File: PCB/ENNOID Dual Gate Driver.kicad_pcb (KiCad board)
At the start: 2 copper layers, 60 x 98 mm, 137 parts, among them J1 Conn_02x08_Odd_Even, J2 Current, J3 TEMP, J4 PHASE, J5 Collector, J6 Gate_H, J7 G_L, J8 E, Q1 Q_NPN_BCE, Q2 Q_NPN_BCE, Q3 2N7002K-7, Q4 2N7002K-7, Q5 2N7002, Q6 2N7002, Q7 2N7002, Q8 2N7002, U1 MC7805, U2 MGJ2, U3 MGJ2, U4 1ED020I12-F2, U5 IXD-609, U6 1ED020I12-F2, U7 IXD-609, U8 AMC1301, U9 4069

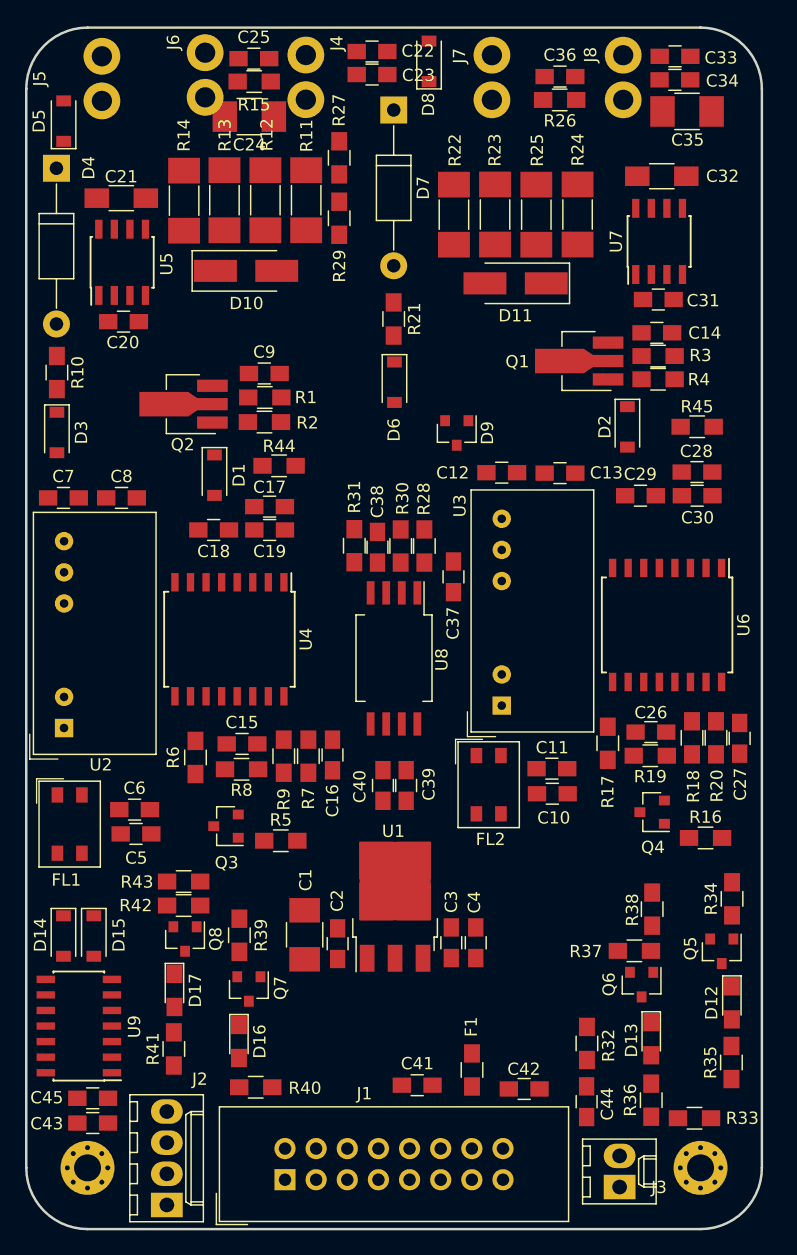
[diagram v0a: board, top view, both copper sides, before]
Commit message: Routing has started
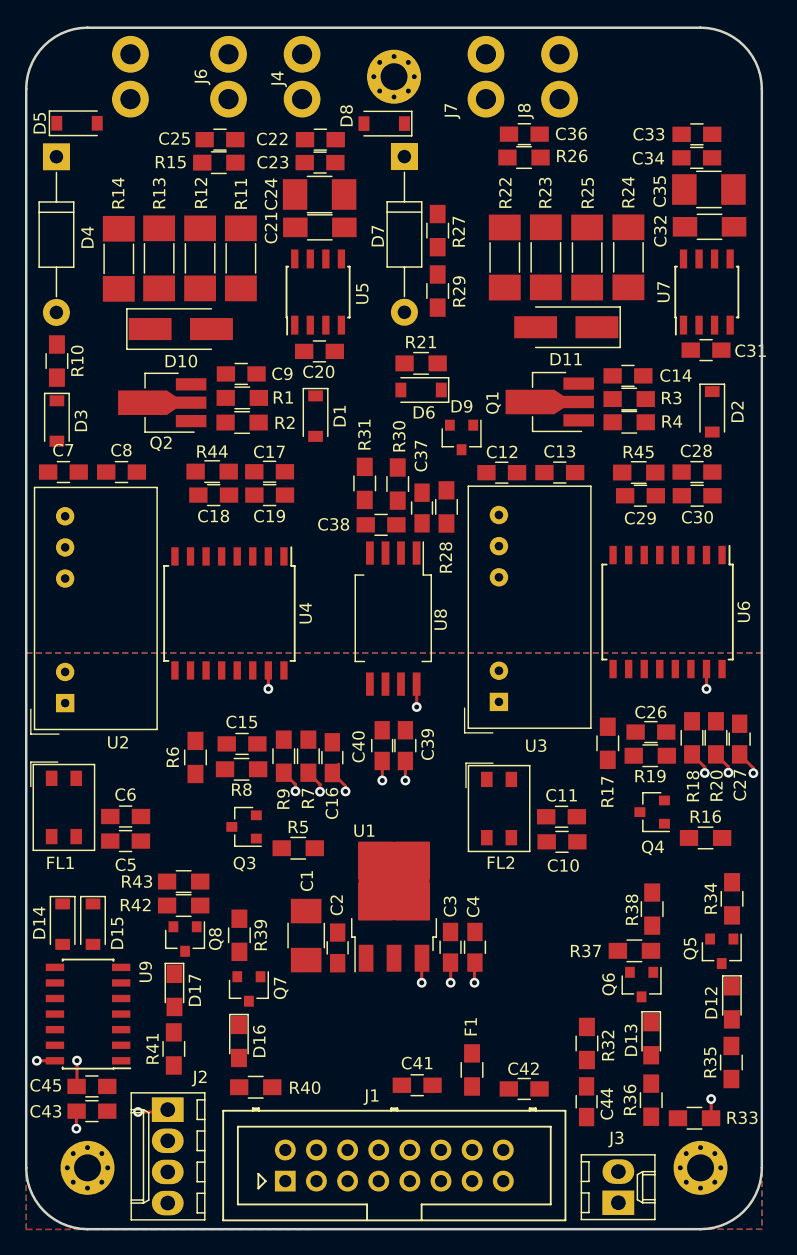
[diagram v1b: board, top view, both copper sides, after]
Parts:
- added REF**: MountingHole_2.2mm_M2_Pad_Via, Mounting_Holes:MountingHole_2.2mm_M2_Pad_Via, F.Cu at (30.0, 4.00)
- J1: footprint Connectors_IDC:IDC-Header_2x08_Pitch2.54mm_Straight -> Connectors_Multicomp:Multicomp_MC9A12-1634_2x08x2.54mm_Straight
- J5: moved to B.Cu
- moved C21 16.4 mm to (23.9, 16.3)
- moved C20 16.2 mm to (23.9, 26.4)
- moved U5 16.2 mm to (23.8, 21.6)
- moved R27 9.99 mm to (33.6, 16.6)
- moved R29 9.99 mm to (33.6, 21.5)
- moved D1 9.55 mm to (23.6, 31.7)
- moved C24 8.56 mm to (23.9, 13.6), turned to 0 degrees
- moved C23 8.34 mm to (24.0, 11.0), turned to 0 degrees
- moved C22 8.34 mm to (24.0, 9.13), turned to 0 degrees
- moved J2 7.77 mm to (11.5, 88.3), turned to 270 degrees
- moved R15 7.22 mm to (15.7, 11.0)
- moved C25 7.16 mm to (15.8, 9.13)
- moved D10 7.13 mm to (12.6, 24.6)
- moved R13 7.13 mm to (10.8, 18.8)
- moved R12 7.13 mm to (14.2, 18.8)
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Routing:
- net +5V: track 0.00 -> 34.9 mm, vias 0 -> 19
- added copper zone on B.Cu, net +5V
- added copper zone on F.Cu, net GND

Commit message: PCB completed with readme update
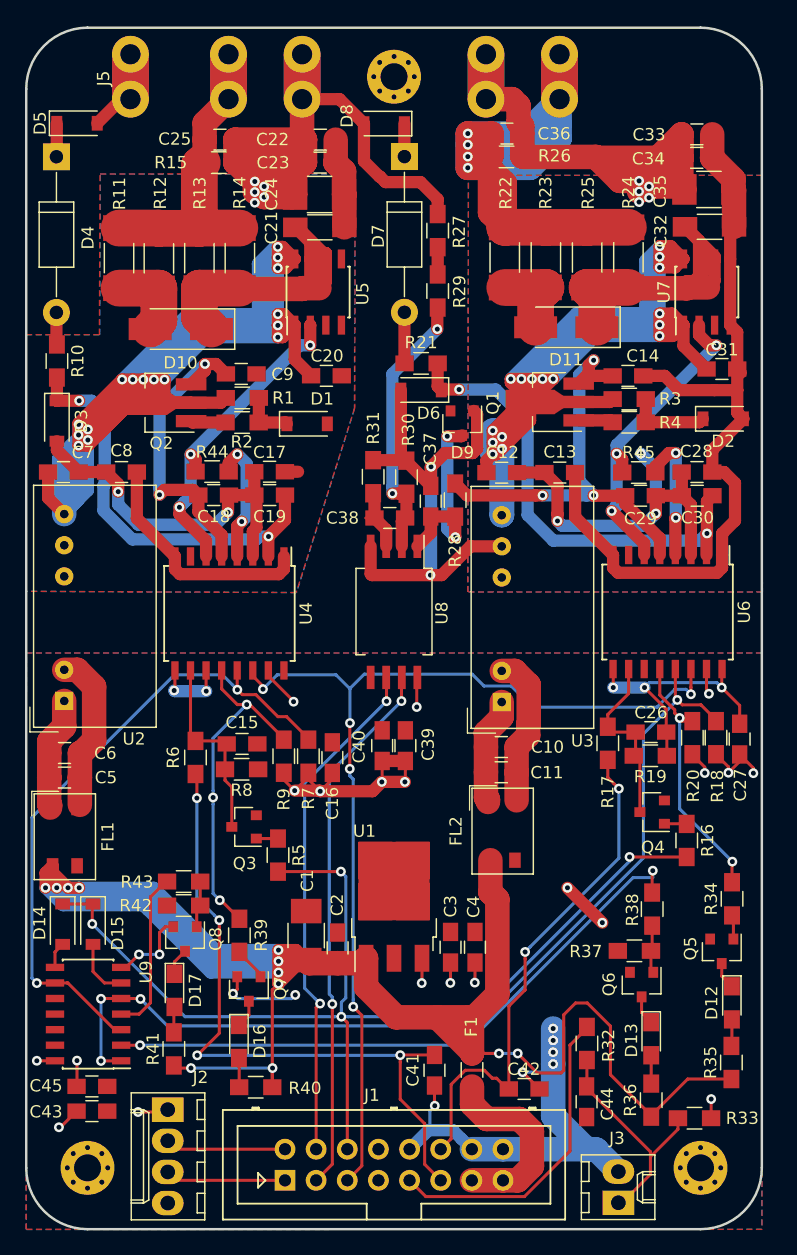
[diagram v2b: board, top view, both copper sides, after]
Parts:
- FL1, FL2: value ACM4520-142-2P-T000 -> ACM4520
- J1: footprint Connectors_Multicomp:Multicomp_MC9A12-1634_2x08x2.54mm_Straight -> ENNOID:Multicomp_MC9A12-1634_2x08x2.54mm_Straight
- J4, J6, J7, J8: moved to B.Cu
- J5: moved to F.Cu
- U8: footprint Housings_SOIC:SSO-8_6.8x5.9mm_Pitch1.27mm_Clearance8mm -> ENNOID:SSO-8_6.8x5.9mm_Pitch1.27mm_Clearance8mm
- moved R11 9.94 mm to (7.57, 18.8)
- moved R14 9.87 mm to (17.4, 18.8)
- moved C10 9.18 mm to (38.7, 58.7), turned to 0 degrees
- moved C5 7.19 mm to (3.12, 61.2)
- moved C6 7.19 mm to (3.13, 59.2)
- moved C11 6.11 mm to (38.7, 60.7), turned to 0 degrees
- moved J7 6.00 mm to (43.5, 4.00), turned to 270 degrees
- moved J8 6.00 mm to (37.5, 4.00), turned to 270 degrees
- moved R12 3.36 mm to (10.8, 18.8)
- moved R13 3.28 mm to (14.1, 18.8)
- moved FL1 2.39 mm to (3.15, 66.0)
- moved C20 2.07 mm to (24.5, 28.4)
- moved C31 2.01 mm to (56.7, 27.8)
- moved R18 1.96 mm to (56.3, 57.9)
- moved R20 1.93 mm to (54.3, 57.9)
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- renumbered REF** to M1, REF** to M2, REF** to M3
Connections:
- FL1 pad 2: Net-(C5-Pad1) -> GND
- FL1 pad 3: GND -> Net-(C5-Pad2)
- FL1 pad 4: Net-(C5-Pad2) -> Net-(C5-Pad1)
- FL2 pad 2: Net-(C10-Pad1) -> GND
- FL2 pad 3: GND -> Net-(C10-Pad2)
- FL2 pad 4: Net-(C10-Pad2) -> Net-(C10-Pad1)
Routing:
- net /GD_HIGH/+VCC: track 0.00 -> 195.4 mm, vias 0 -> 16
- net VCC_IN: track 0.00 -> 192.6 mm, vias 0 -> 12
- net /GD_LOW/+VCC: track 0.00 -> 167.7 mm, vias 0 -> 16
- net /GD_LOW/E: track 0.00 -> 123.8 mm, vias 0 -> 10
- net FLT_ALL: track 0.00 -> 89.7 mm, vias 0 -> 4
- net PHASE: track 0.00 -> 87.9 mm, vias 0 -> 7
- net RST: track 0.00 -> 83.2 mm, vias 0 -> 5
- net GND: track 0.00 -> 80.5 mm, vias 0 -> 15
- net FLT_L: track 0.00 -> 78.1 mm, vias 0 -> 4
- net /GD_LOW/G: track 0.00 -> 69.2 mm, vias 0 -> 4
- net /GD_LOW/-VEE: track 0.00 -> 66.3 mm
- net PWM_H: track 0.00 -> 55.4 mm, vias 0 -> 4
- net FLT_H: track 0.00 -> 54.3 mm, vias 0 -> 2
- net Net-(R38-Pad1): track 0.00 -> 51.4 mm, vias 0 -> 2
- net Vout+: track 0.00 -> 44.1 mm, vias 0 -> 2
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- added copper zone on F.Cu, net /GD_HIGH/-VEE
- added copper zone on F.Cu, net /GD_LOW/-VEE
- added copper zone on B.Cu, net /GD_LOW/E
- added copper zone on B.Cu, net PHASE
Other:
- board text added: "E1"
- board text added: "E2"
- board text added: "G1"
- board text added: "G2"

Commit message: Minor updates
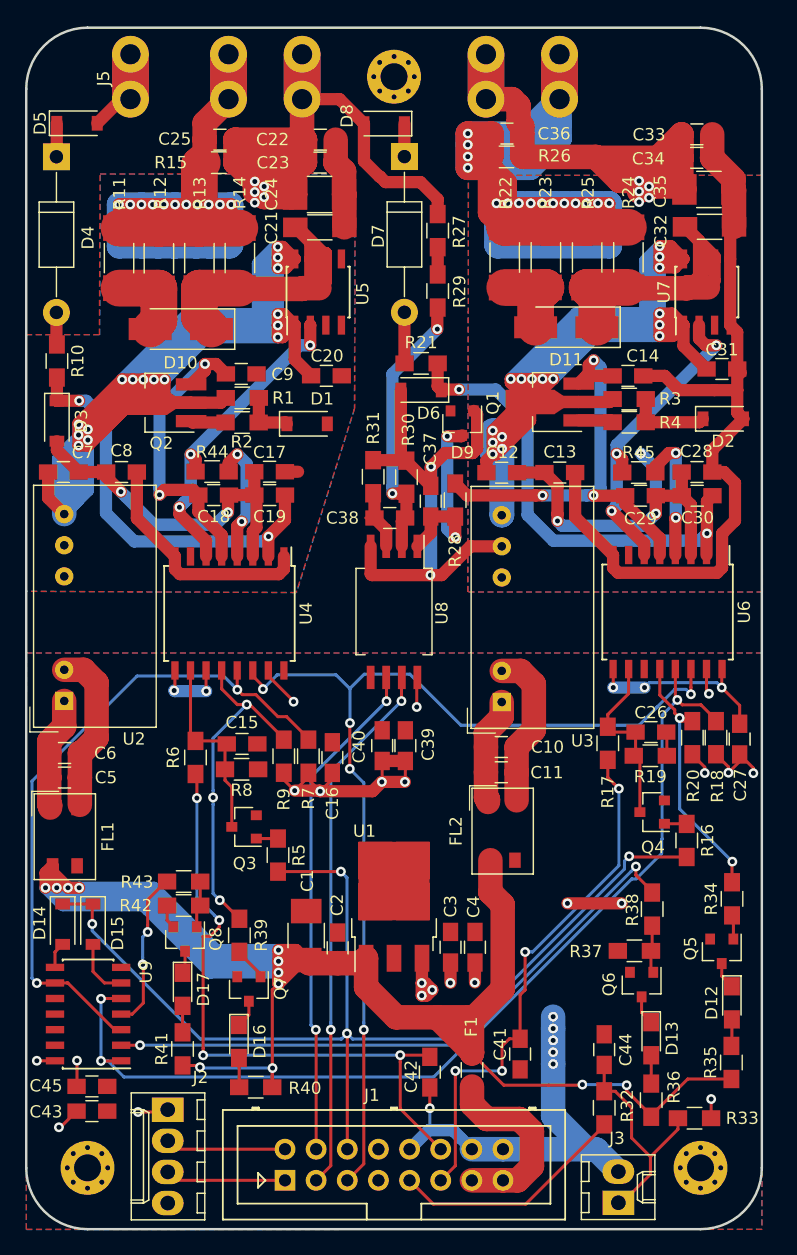
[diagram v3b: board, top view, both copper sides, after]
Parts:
- moved C42 7.82 mm to (32.9, 85.2), turned to 270 degrees
- moved C41 7.11 mm to (40.3, 83.7)
- moved R32 5.44 mm to (47.1, 88.1), turned to 270 degrees
- moved C44 4.49 mm to (47.1, 83.4), turned to 90 degrees
- moved R41 0.71 mm to (12.8, 83.3)
- moved D17 0.67 mm to (12.8, 78.4)
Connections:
- C41 pad 1: PWM_H -> PWM_L
- C42 pad 1: PWM_L -> PWM_H
- J1 pad 11: PWM_H -> PWM_L
- J1 pad 12: PWM_L -> PWM_H
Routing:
- net /GD_LOW/G: track 69.2 -> 144.7 mm, vias 4 -> 15
- net /GD_HIGH/G: track 28.7 -> 93.5 mm, vias 0 -> 11
- net GND: track 80.5 -> 62.2 mm, vias 15 -> 11
- net VCC_IN: track 192.6 -> 182.9 mm
- net TEMP: track 25.9 -> 19.4 mm
- net FLT_L: track 78.1 -> 81.8 mm, vias 4 -> 3
- net +5V: track 58.2 -> 61.7 mm, vias 20 -> 22
- net PWM_H: track 55.4 -> 52.2 mm
- net FLT_ALL: track 89.7 -> 91.8 mm
- net PWM_L: track 42.4 -> 44.0 mm, vias 2 -> 4
- net FLT_H: track 54.3 -> 55.9 mm
- net RST: track 83.2 -> 84.5 mm
- net PHASE: track 87.9 -> 87.2 mm
- net Net-(R38-Pad1): track 51.4 -> 50.7 mm
- net Vout-: track 41.9 -> 41.2 mm
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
